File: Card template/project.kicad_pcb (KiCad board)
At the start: 2 copper layers, 51.5 x 22 mm, 3 parts, among them U1 24LC32, X0 Card Edge

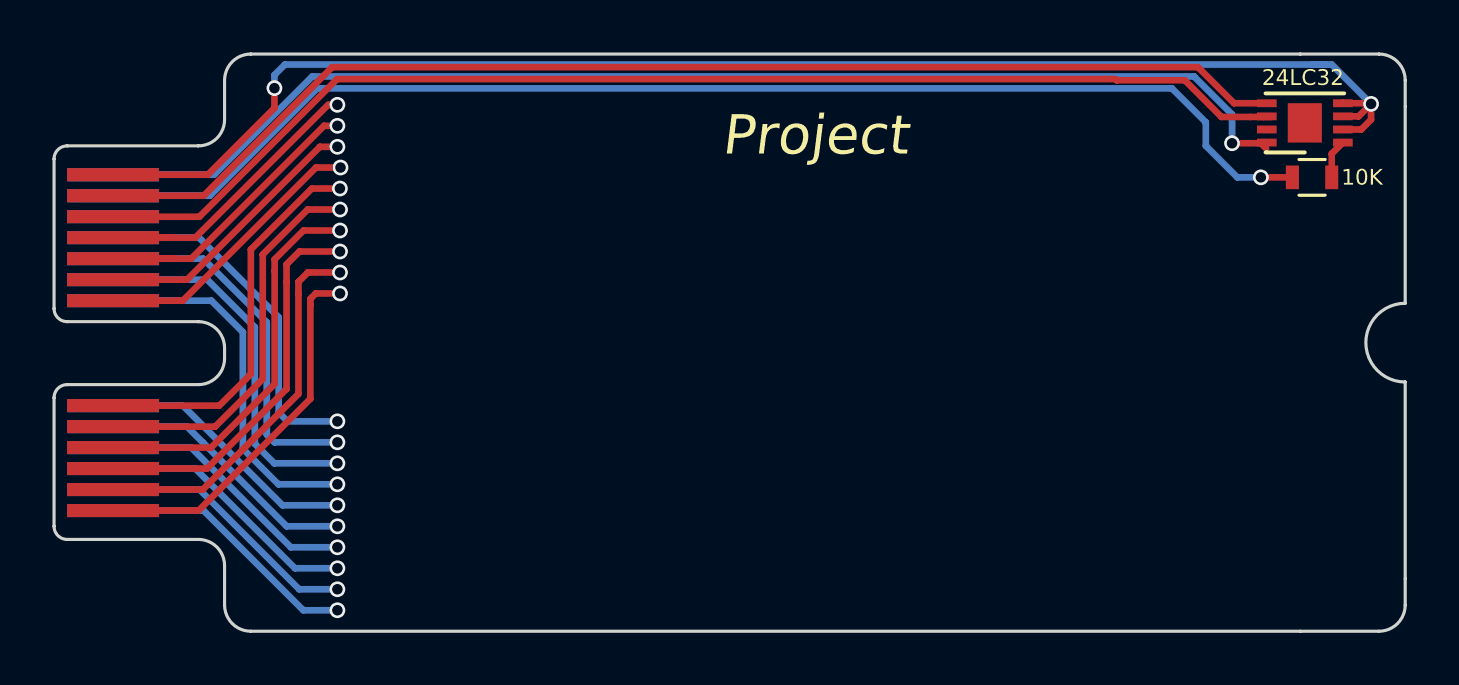
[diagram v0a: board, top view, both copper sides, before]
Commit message: Updates
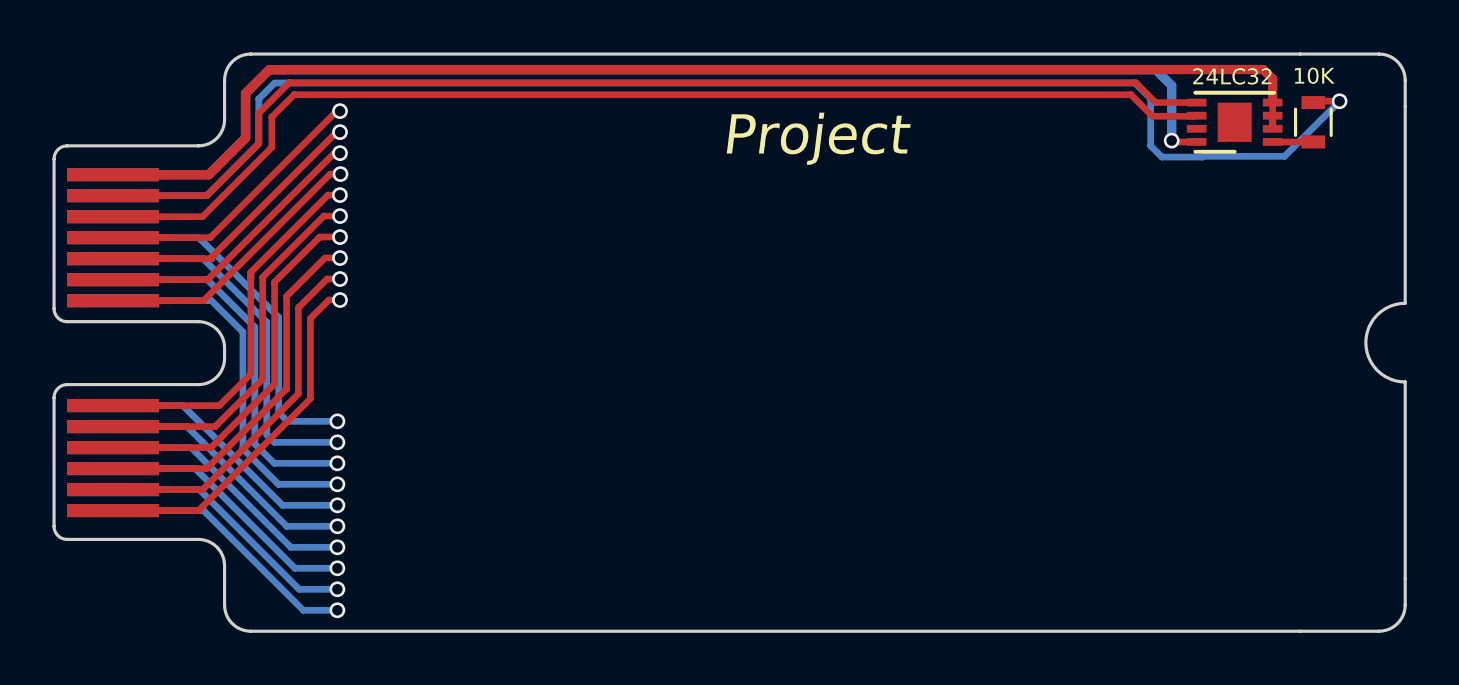
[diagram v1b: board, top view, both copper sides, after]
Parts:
- moved U1 2.68 mm to (45.0, -18.5)
- moved R1 2.10 mm to (48.0, -18.5), turned to 90 degrees
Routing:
- net GND: track 55.8 -> 49.2 mm, vias 2 -> 0
- net /A: track 48.6 -> 53.7 mm
- net /19: track 13.0 -> 16.0 mm
- net /D3_SCL: track 46.9 -> 44.3 mm
- net /D2_SDA: track 46.6 -> 44.1 mm
- net +5V: track 47.3 -> 46.3 mm
- net /13: track 14.9 -> 14.0 mm
- net /12: track 14.6 -> 13.9 mm
- net /15: track 14.9 -> 14.2 mm
- net /14: track 14.9 -> 14.2 mm
- net /11: track 14.5 -> 13.9 mm
